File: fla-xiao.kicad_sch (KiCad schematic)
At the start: 9 parts, among them J1 Conn_PinHeader_1x08_P2.54mm_V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, J2 Conn_PinHeader_1x04_P2.54mm_V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, J3 Conn_PinHeader_2x03_P2.54mm_V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, M1 Module_XIAO-RP2040_SocketSMD, SW1 BUTTON_B3SN

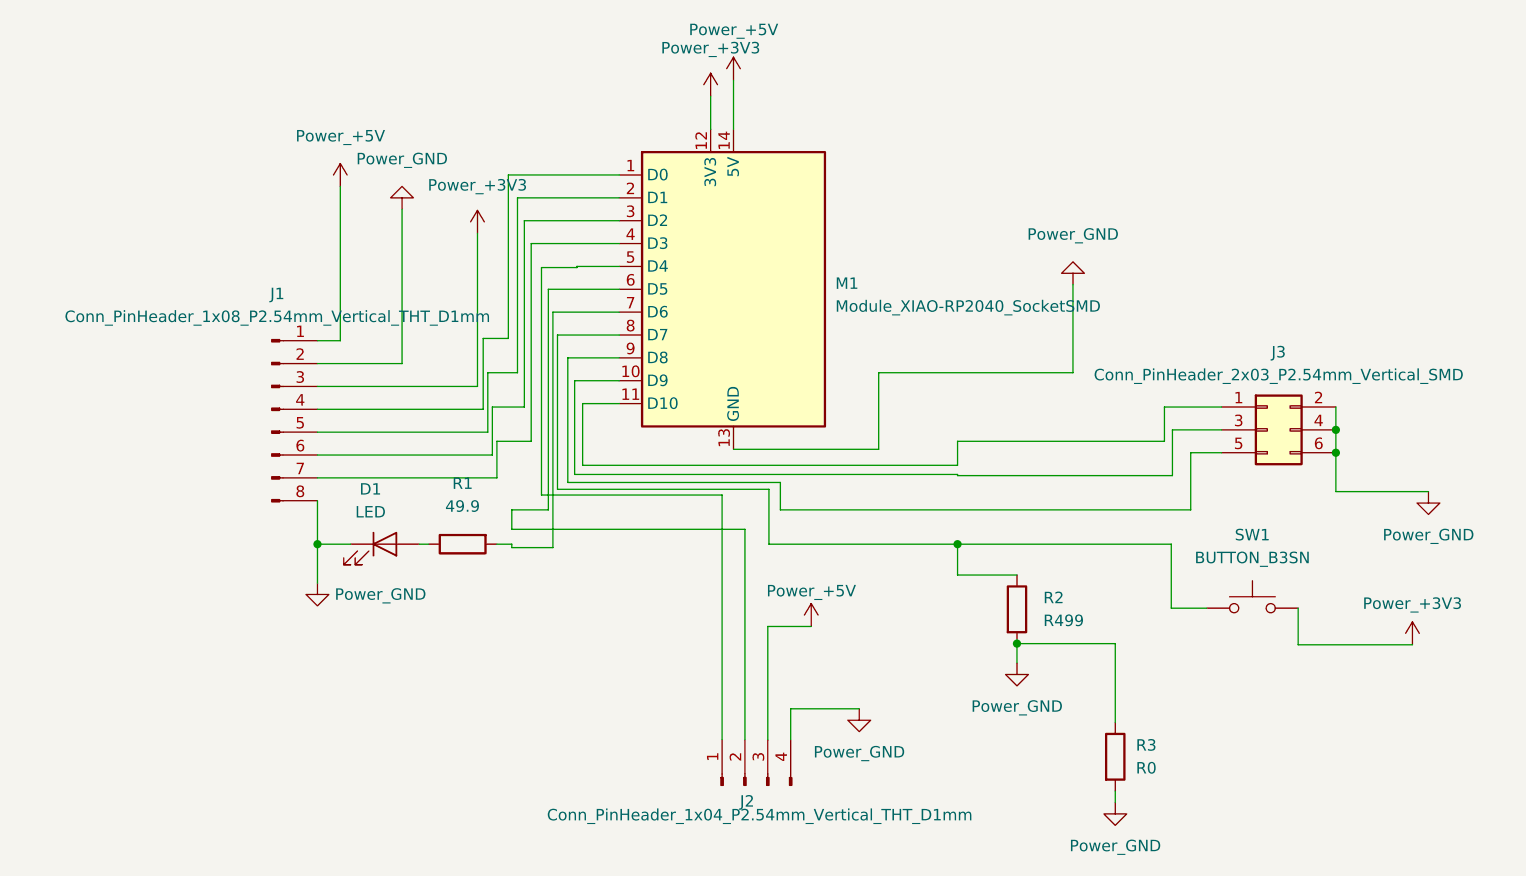
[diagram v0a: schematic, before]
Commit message: Updated board
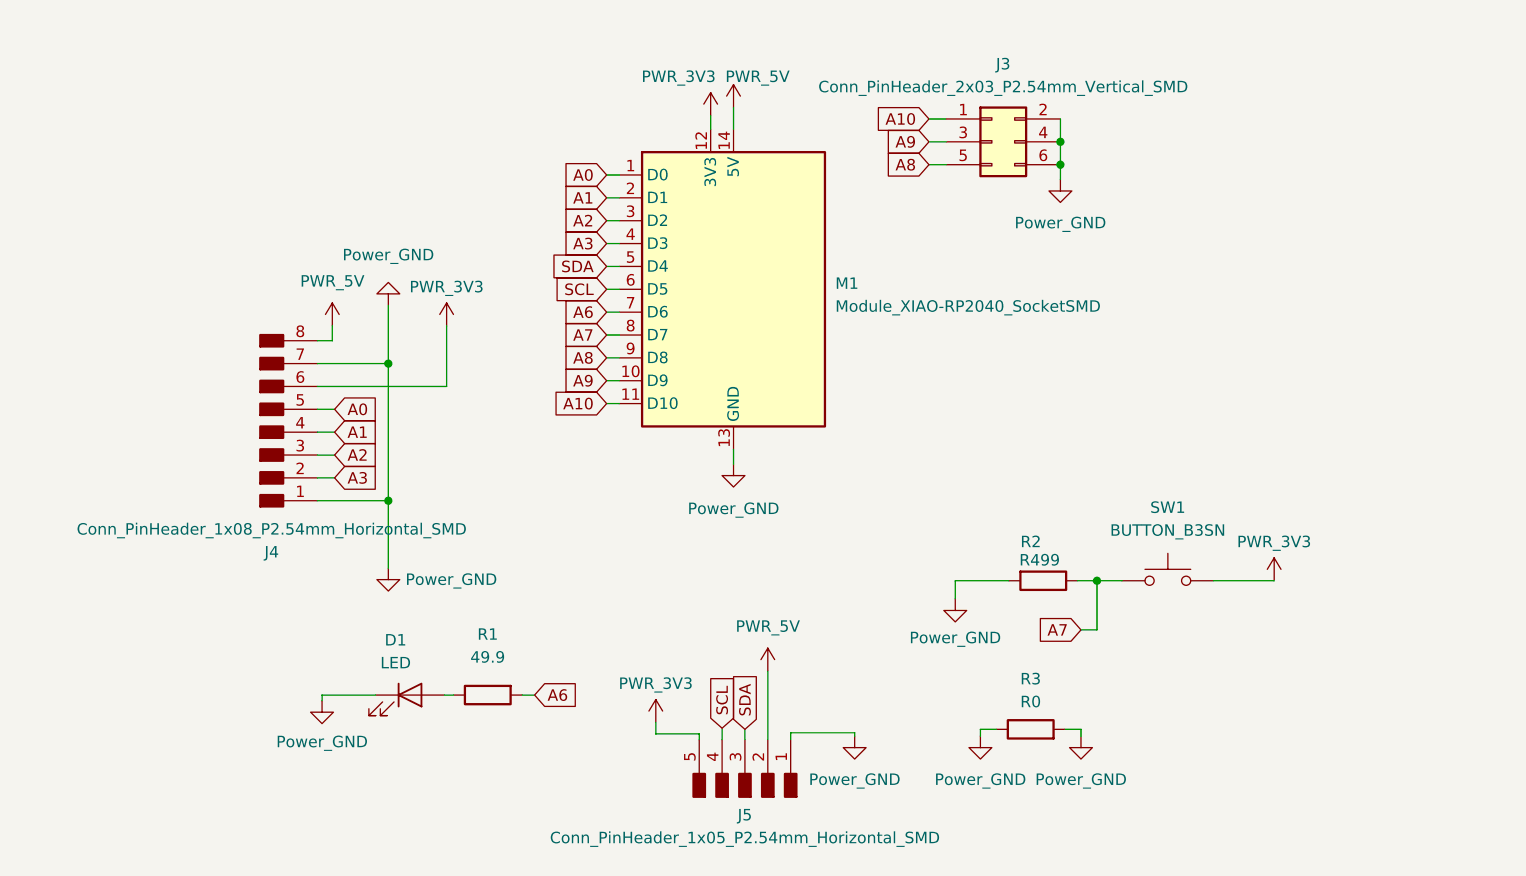
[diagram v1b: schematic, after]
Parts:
- removed J1: Conn_PinHeader_1x08_P2.54mm_Vertical_THT_D1mm, fab:PinHeader_1x08_P2.54mm_Vertical_THT_D1mm, symbol fab:Conn_PinHeader_1x08_P2.54mm_Vertical_THT_D1mm
- removed J2: Conn_PinHeader_1x04_P2.54mm_Vertical_THT_D1mm, fab:PinHeader_1x04_P2.54mm_Vertical_THT_D1mm, symbol fab:Conn_PinHeader_1x04_P2.54mm_Vertical_THT_D1mm
- added J4: Conn_PinHeader_1x08_P2.54mm_Horizontal_SMD, fab:PinHeader_1x08_P2.54mm_Horizontal_SMD, symbol fab:Conn_PinHeader_1x08_P2.54mm_Horizontal_SMD
- added J5: Conn_PinHeader_1x05_P2.54mm_Horizontal_SMD, fab:PinHeader_1x05_P2.54mm_Horizontal_SMD, symbol fab:Conn_PinHeader_1x05_P2.54mm_Horizontal_SMD
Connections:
- net GND: now also J4.1 (Pin_1), J4.7 (Pin_7), J5.1 (Pin_1)
- net A7: now reaches M1.8 (D7), R2.1, SW1.1
- net A0: now reaches M1.1 (D0)
- net A0: now also J4.5 (Pin_5)
- net A1: now reaches M1.2 (D1)
- net A1: now also J4.4 (Pin_4)
- net A2: now reaches M1.3 (D2)
- net A2: now also J4.3 (Pin_3)
- net A3: now reaches M1.4 (D3)
- net A3: now also J4.2 (Pin_2)
- net A9: now reaches J3.3 (Pin_3), M1.10 (D9)
- net A10: now reaches J3.1 (Pin_1), M1.11 (D10)
- net SDA: now reaches M1.5 (D4)
- net SDA: now also J5.3 (Pin_3)
- net SCL: now reaches M1.6 (D5)
- net SCL: now also J5.4 (Pin_4)
- net A6: now reaches M1.7 (D6), R1.2
- net A8: now reaches J3.5 (Pin_5), M1.9 (D8)
- net +3V3 renamed PWR_3V3
- net PWR_3V3: now also J4.6 (Pin_6), J5.5 (Pin_5)
- net +5V renamed PWR_5V
- net PWR_5V: now also J4.8 (Pin_8), J5.2 (Pin_2)
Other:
- moved on the sheet: D1, J3, R1, R2, R3, SW1
